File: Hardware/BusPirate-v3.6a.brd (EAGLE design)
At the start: 53.3 x 30.5 mm, 50 parts, among them IC1 PIC24FJ64GA002-I/SSSS-ALTERNA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, IC2 FT232RLSSOP, IC3 4066D, J1 USBSMD

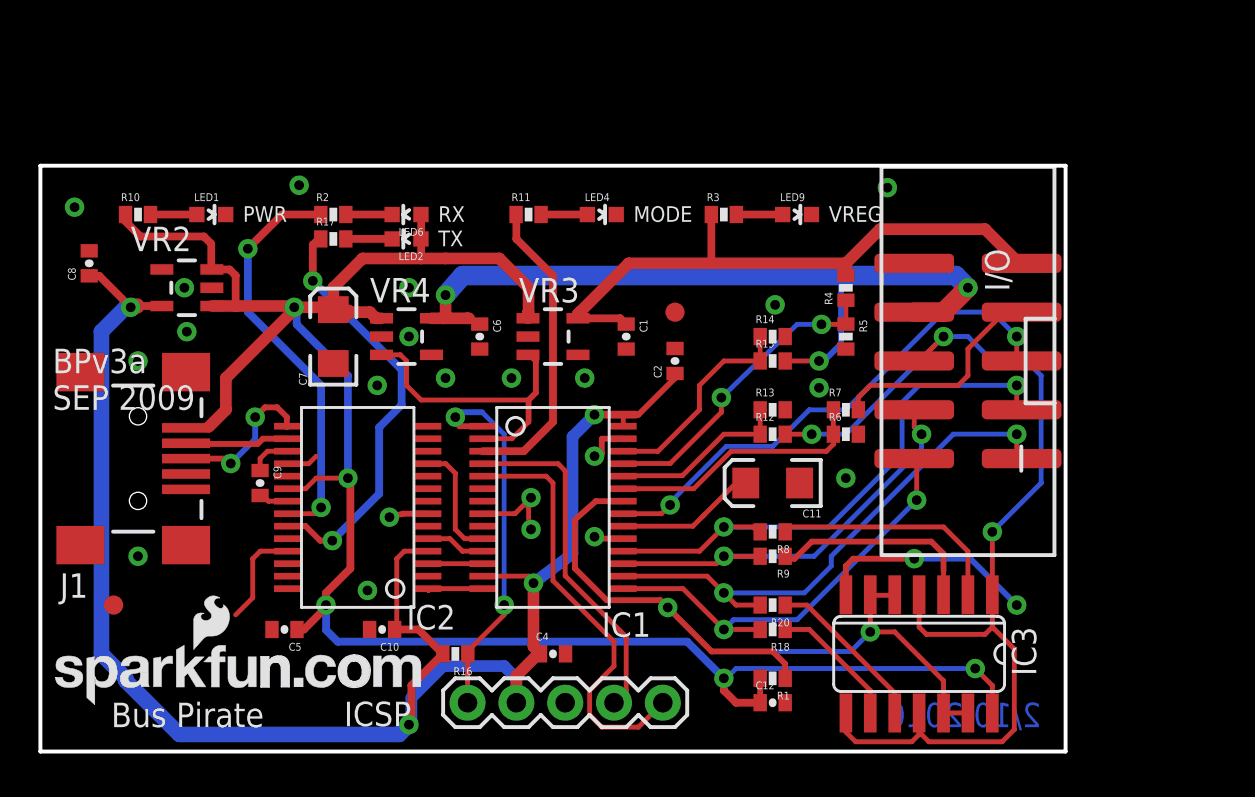
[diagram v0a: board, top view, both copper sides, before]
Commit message: First commit of v3.6a
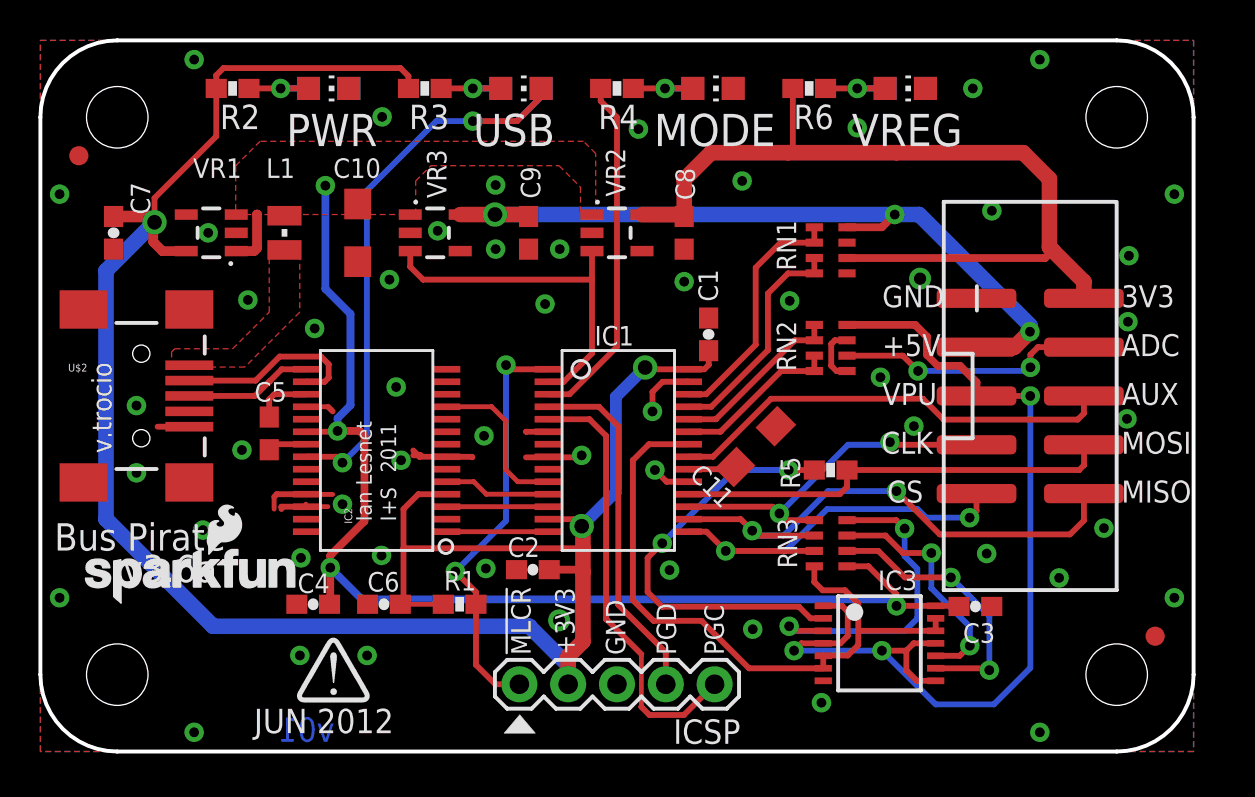
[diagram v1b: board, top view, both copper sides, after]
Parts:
- removed C12: 0.1uF, SparkFun:0402-CAP
- removed I/O: M05X2SHD_SMD, SparkFun:2X5-SHROUDED_SMD
- removed J1: USBSMD, SparkFun:USB-MINIB
- removed JP2: LOGO-SFENEW, SparkFun:SFE-NEW-WEBLOGO
- removed JP3, JP4: FIDUCIAL1X2, SparkFun:FIDUCIAL-1X2
- removed LED6: BLUE, SparkFun:LED-0603
- removed LED9: YELLOW, SparkFun:LED-0603
- removed R10, R17: 1k1, SparkFun:0402-RES
- removed R11: 390R, SparkFun:0402-RES
- removed R12, R13, R14, R15, R18, R20, R7, R9: 10k, SparkFun:0402-RES
- removed R16, R8: 2k, SparkFun:0402-RES
- removed VR4: 5V, SparkFun:SOT23-5
- added C3: 0.1uF, SparkFun-Capacitors:0603-CAP
- added FID1, FID2: FIDUCIAL1X2, SparkFun-Aesthetics:FIDUCIAL-1X2
- added FRAME1: FRAME-LETTER, SparkFun-Aesthetics:CREATIVE_COMMONS
- added L1: 700mA+ ferrite, wuerth-elektronik:WE-KI_0805_B
- added LED1A, LED2A, LED3, LED3A, LED4A: (no value), led:CHIP-LED0805
- added LOGO1: SFE_LOGO_NAME_FLAME.1_INCH, SparkFun-Aesthetics:SFE_LOGO_NAME_FLAME_.1
- added LOGO2: OSHW-LOGOL, SparkFun-Aesthetics:OSHW-LOGO-L
- added RN1, RN2, RN3: 10k, Testing:4XARRAY
- added U$3: (no value), dp_devices:DP_LOGO_ART_1X1
- added VR1: MIC5205 3V3, SparkFun-PowerIC:SOT23-5
- C1, C6: value 2.2uF -> 0.1uF; device SparkFun:0402-CAP -> SparkFun-Capacitors:0603-CAP
- C10: value 0.1uF -> 10uF; device SparkFun:0402-CAP -> rcl:SMC_A
- C11: device SparkFun:EIA3216 -> rcl:SMC_A
- C2, C4: device SparkFun:0402-CAP -> SparkFun-Capacitors:0603-CAP
- C5: device SparkFun:0402-CAP -> dp_devices:C603
- C7: value 10uF -> 0.1uF; device SparkFun:EIA3216 -> SparkFun-Capacitors:0603-CAP
- C8: value 2.2uF -> 1uF; device SparkFun:0402-CAP -> dp_devices:C603
- C9: value 0.1uF -> 1uF; device SparkFun:0402-CAP -> dp_devices:C603
- IC1: value PIC24FJ64GA002-I/SSSS-ALTERNATE -> PIC24FJ64GA002; device microchip-pic24:SSOP28DB -> dp_devices:SSOP28
- IC2: value FT232RLSSOP -> FT232RL-BASICSSOP; device SparkFun:SSOP28DB -> SparkFun-DigitalIC:SSOP28DB
- IC3: value 4066D -> 4066; device 40xx:SO14 -> 40xx:TSSOP14
- ICSP: value M05X1PTH -> (none); device SparkFun:1X05 -> SparkFun-Connectors:1X05
- JP1: value LOGO-SFENEW -> (none); device SparkFun:SFE-NEW-WEBLOGO -> SparkFun-Connectors:2X5-SHROUDED_SMD
- LED1, LED4: value RED -> (none); device SparkFun:LED-0603 -> led:CHIP-LED0805
- LED2: value GREEN -> (none); device SparkFun:LED-0603 -> led:CHIP-LED0805
- R1, R5: value 10k -> 2.0k; device SparkFun:0402-RES -> SparkFun-Resistors:0603-RES
- R2: value 1k1 -> 1K; device SparkFun:0402-RES -> SparkFun-Resistors:0603-RES
- R3: value 390R -> 1K; device SparkFun:0402-RES -> SparkFun-Resistors:0603-RES
- R4, R6: value 10k -> 1K; device SparkFun:0402-RES -> SparkFun-Resistors:0603-RES
- U$2: value CREATIVE_COMMONS -> USB-MINIB-5PIN; device SparkFun:CREATIVE_COMMONS -> SparkFun-Connectors:USB-MINIB
- VR2: value 3.3V -> MIC5205 3V3; device SparkFun:SOT23-5 -> SparkFun-PowerIC:SOT23-5
- VR3: value 3.3V -> MIC5205 5V0; device SparkFun:SOT23-5 -> SparkFun-PowerIC:SOT23-5
- moved JP1 53.2 mm to (51.5, 18.5)
- moved C8 31.0 mm to (33.5, 27.0), turned to 270 degrees
- moved U$2 30.1 mm to (5.25, 18.5)
- moved U$1 25.6 mm to (13.3, 2.54), flipped to the top
- moved VR2 22.6 mm to (30.0, 27.0), turned to 270 degrees
- moved C10 20.7 mm to (16.5, 27.0), turned to 270 degrees
- moved C9 19.1 mm to (25.4, 27.0)
- moved R6 18.1 mm to (40.0, 34.5), turned to 180 degrees
- moved LED2 17.8 mm to (35.0, 34.5), turned to 270 degrees
- moved R3 16.9 mm to (20.0, 34.5), turned to 180 degrees
- moved R1 16.7 mm to (21.8, 7.66)
- moved R4 15.8 mm to (30.0, 34.5), turned to 180 degrees
- moved C6 14.8 mm to (17.9, 7.66), turned to 180 degrees
- moved C2 13.1 mm to (25.6, 9.46), turned to 180 degrees
- moved ICSP 12.9 mm to (35.1, 3.50), turned to 180 degrees
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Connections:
- removed net MCLR: IC1.1, ICSP.1, R16.1
- removed net N$10: LED2.C, R17.2
- removed net N$11: IC2.22, R2.1
- removed net N$15: IC2.15, J1.D+
- removed net N$16: IC2.16, J1.D-
- removed net N$8: IC2.23, R17.1
- removed net SWV33: C1.1, I/O.9, R3.1, R4.2, VR3.5
- removed net SWV50: C6.1, I/O.8, R15.2, VR4.5
- removed net TP1: IC1.7
- removed net TP2: IC1.6
- removed net V+: C12.1, C5.1, C7.A, IC2.20, IC3.14, J1.VBUS, LED2.A, LED6.A, R1.2, R10.1, VR2.1, VR2.3, VR3.1, VR4.1
- new net !MCLR: IC1.1, ICSP.5, R1.1
- new net $N26: L1.2, U$2.VBUS
- new net 5V: C10.+, C3.1, C4.1, IC2.20, IC3.14, L1.1, RN3.5, VR1.1, VR1.3, VR2.1, VR3.1
- new net D+: IC2.15, U$2.D+
- new net D-: IC2.16, U$2.D-
- new net RXLED: IC2.22, LED4.C, LED4A.C
- new net SW3V3: C8.1, JP1.2, R6.2, RN1.6, VR2.5
- new net SW5V0: C9.1, JP1.3, RN1.8, VR3.5
- net ADC: now also JP1.4, RN2.6; no longer I/O.7, R7.2
- net ADC1: now also RN2.3, RN2.4; no longer R6.1, R7.1
- net ADC2: now also RN2.1, RN2.2; no longer R12.1, R13.1
- net ADC3: now also RN1.3, RN1.4; no longer R4.1, R5.1
- net ADC4: now also RN1.1, RN1.2; no longer R14.1, R15.1
- net AUX1: now also JP1.6; no longer I/O.5
- net CLK: now also JP1.7, RN3.1; no longer I/O.4, R9.2
- net CS: now also JP1.9, RN3.3; no longer I/O.2, R18.2
- net GND: now also C10.-, C11.-, C3.2, C7.2, IC1.6, IC1.7, JP1.1, LED1A.C, LED2.C, LED2A.C, LED3.C, LED3A.C, RN1.5, RN1.7, RN2.5, RN2.7, U$2.GND, VR1.2; no longer C10.2, C11.C, C12.2, C7.C, I/O.10, J1.GND, LED4.C, LED9.C, R13.2, R14.2, R5.2, R6.2, VR4.2
- net LD1: now also R4.2; no longer R11.1
- net MISO: now also JP1.10, RN3.2; no longer I/O.1, R20.2
- net MOSI: now also JP1.8, R5.1; no longer I/O.3, R8.2
- net N$1: now also R5.2; no longer R8.1
- net N$13: now also LED4.A, LED4A.A, R3.1; no longer LED6.C, R2.2
- net N$18: now also LED3.A, LED3A.A, R6.1; no longer LED9.A, R3.2
- net N$2: now also IC3.9, RN3.6; no longer IC3.3, R9.1
- net N$3: now also C11.+; no longer C11.A
- net N$4: now also RN3.7; no longer R20.1
- net N$5: now also IC3.3, RN3.8; no longer IC3.9, R18.1
- net N$6: now also LED2.A, LED2A.A, R4.1; no longer LED4.A, R11.2
- net N$7: now also LED1A.A, R2.1; no longer R10.2
- net N$9: now also C5.1; no longer C9.1
- net PGC: now also ICSP.1; no longer ICSP.5
- net PGD: now also ICSP.2; no longer ICSP.4
- net PULLUPEN: now also RN3.4; no longer R1.1
- net VCC: now also C1.1, C6.1, C7.1, ICSP.4, R1.2, R2.2, R3.2, VR1.5; no longer C10.1, C4.1, C8.1, ICSP.2, R16.2, VR2.5
- net VEXTERN: now also JP1.5, RN2.8; no longer I/O.6, R12.2
- net VREGEN: now also VR2.3; no longer VR4.3
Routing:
- net V+: track 111.2 -> 0.00 mm, vias 5 -> 0
- net 5V: track 0.00 -> 66.5 mm, vias 0 -> 4
- net SW3V3: track 0.00 -> 45.7 mm
- net SWV50: track 42.2 -> 0.00 mm, vias 3 -> 0
- net SW5V0: track 0.00 -> 40.2 mm, vias 0 -> 3
- net RXLED: track 0.00 -> 32.7 mm, vias 0 -> 2
- net SWV33: track 32.2 -> 0.00 mm
- net VCC: track 89.8 -> 115.1 mm, vias 4 -> 3
- net !MCLR: track 0.00 -> 22.1 mm, vias 0 -> 2
- net N$8: track 22.0 -> 0.00 mm, vias 2 -> 0
- net N$11: track 21.5 -> 0.00 mm, vias 2 -> 0
- net MCLR: track 19.8 -> 0.00 mm, vias 2 -> 0
- net D-: track 0.00 -> 9.90 mm
- net N$5: track 7.16 -> 17.1 mm, vias 0 -> 2
- net N$1: track 12.5 -> 22.1 mm, vias 0 -> 2
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- added copper zone on layer 1, net $N26
- added copper zone on layer 1, net 5V
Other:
- board size 53.3 x 30.5 mm -> 60 x 37 mm
- board text added: "!MLCR"
- board text added: "+3V3"
- board text added: "2011"
- board text added: "3V3"
- board text added: "All units in mm"
- board text added: "BPv3.6a"
- board text added: "I+S"
- board text added: "Ian Lesnet http://dangerousprototypes.com"
- board text added: "JUN 2012"
- board text added: "Revised by: Brent Wilkins (Based on BP v3.6a)"
- board text added: "VPU"
- board text added: "v.trocio"
- board text added: "v01"
- board text added: "v3.6a"
- board text removed: "+3.3V"
- board text removed: "+3v"
- board text removed: "+5v"
- board text removed: "2/10/2010"
- board text removed: "AUX1"
- board text removed: "BPv3"
- board text removed: "BPv3a"
- board text removed: "Based on design by"
- board text removed: "CLOCK"
- board text removed: "DATA"
- board text removed: "DangerousPrototypes.com"
- board text removed: "Fulfillment by"
- board text removed: "ICSP"
- board text removed: "Layout for SparkFun Electronics by Chris Taylor"
- board text removed: "RX"
- board text removed: "SEP 2009"
- board text removed: "Seeed Studio"
- board text removed: "TX"
- board text removed: "VCC"
- board text removed: "Vpu"
- board text removed: "dangerousprototypes.com"
- board text removed: "www.seeedstudio.com"
